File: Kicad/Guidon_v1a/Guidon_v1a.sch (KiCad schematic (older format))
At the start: 0 parts

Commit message: Update Schematic
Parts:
- added C1: 10u, symbol Device:CP1
- added C10, C11, C12, C5, C6, C7, C8, C9: 680n, symbol Device:C
- added C2: 100u, symbol Device:CP1
- added C3, C4: 100n, symbol Device:C
- added D1: D_Schottky_AKA, symbol Device:D_Schottky_AKA
- added IC1: R-785.0-0.5, RECOM_R-785.0-0.5, symbol R-785.0-0.5:R-785.0-0.5
- added IC2: MCP2562, Package_SO:SOIC-8_3.9x4.9mm_P1.27mm, symbol Interface_CAN_LIN:MCP2562-E-SN
- added K1: ALIM, symbol Connector_Generic:Conn_01x02
- added K2: BUS CAN, symbol Connector_Generic:Conn_01x02
- added K3: INTER., symbol Connector_Generic:Conn_01x09
- added K4: OLED, symbol Connector_Generic:Conn_01x04
- added R1: 120, symbol Device:R
- added R10, R2, R3, R4, R5, R6, R7, R8: 6.8k, symbol Device:R
- added R11, R9: 3.3k, symbol Device:R
- added UC1: BluePill STM32, symbol YAAJ_STM32:BluePill_1
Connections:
- new net: IC2.6 (CANL), K2.2 (Pin_2), R1.2
- new net: IC2.7 (CANH), K2.1 (Pin_1), R1.1
- new net: C1.1, D1.2 (K), IC1.1 (+VIN)
- new net: D1.1 (A), D1.3 (A), K1.1 (Pin_1)
- new net +5V: C2.1, C4.2, IC1.3 (+VOUT), IC2.3 (VDD), UC1.18 (5V)
- new net BP0: C5.1, K3.1 (Pin_1), R2.2, UC1.25 (PA0)
- new net BP1: C6.1, K3.2 (Pin_2), R3.2, UC1.26 (PA1)
- new net BP2: C7.1, K3.3 (Pin_3), R4.2, UC1.27 (PA2)
- new net BP3: C8.1, K3.4 (Pin_4), R5.2, UC1.28 (PA3)
- new net BP4: C9.1, K3.5 (Pin_5), R6.2, UC1.29 (PA4)
- new net BP5: C10.1, K3.6 (Pin_6), R7.2, UC1.30 (PA5)
- new net BP6: C11.1, K3.7 (Pin_7), R8.2, UC1.31 (PA6)
- new net BP7: C12.1, K3.8 (Pin_8), R10.2, UC1.32 (PA7)
- new net CANRX: IC2.4 (RXD), UC1.8 (PA11)
- new net CANTX: IC2.1 (TXD), UC1.9 (PA12)
- new net GND: C1.2, C10.2, C11.2, C12.2, C2.2, C3.2, C4.1, C5.2, C6.2, C7.2, C8.2, C9.2, IC1.2 (GND), IC2.2 (VSS), IC2.8 (STBY), K1.2 (Pin_2), K3.9 (Pin_9), K4.2 (Pin_2), UC1.19 (GND), UC1.39 (GND), UC1.40 (GND)
- new net SCL: K4.3 (Pin_3), R11.2, UC1.14 (PB6)
- new net SDA: K4.4 (Pin_4), R9.2, UC1.15 (PB7)
- new net VCC: C3.1, IC2.5 (Vio), K4.1 (Pin_1), R10.1, R11.1, R2.1, R3.1, R4.1, R5.1, R6.1, R7.1, R8.1, R9.1, UC1.20 (3V3)
- no-connect marks 0 -> 23

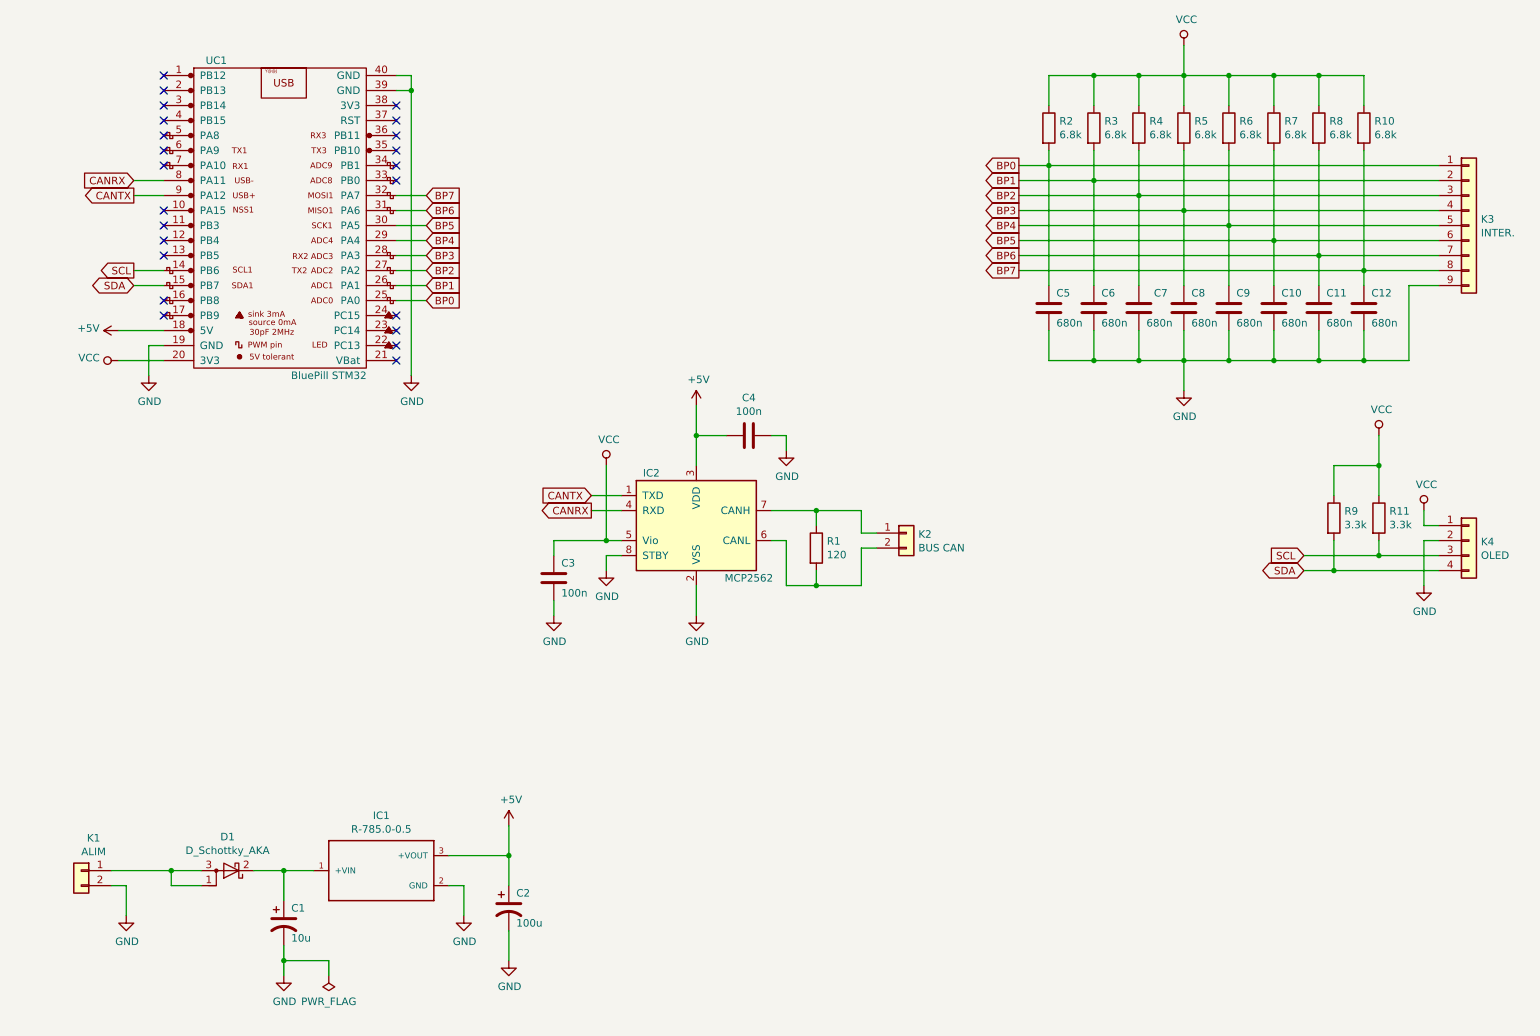
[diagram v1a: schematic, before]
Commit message: Update projet
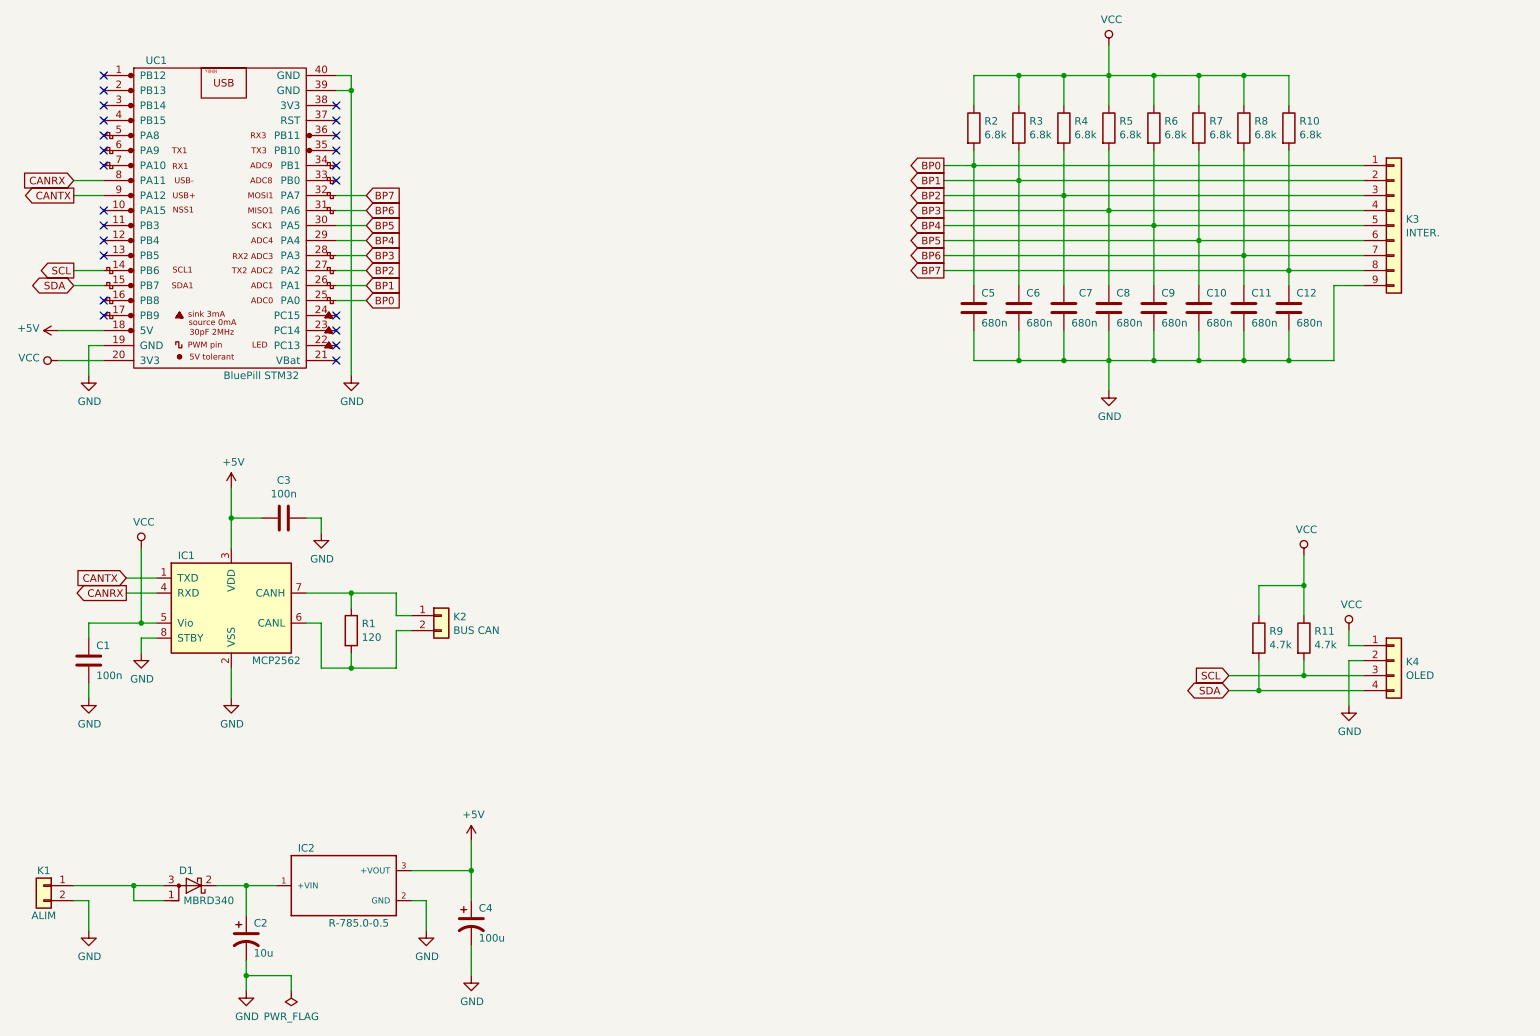
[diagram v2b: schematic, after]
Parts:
- D1: value D_Schottky_AKA -> MBRD340
- R11, R9: value 3.3k -> 4.7k
- renumbered C3 to C1, C1 to C2, C4 to C3, C2 to C4, IC2 to IC1, IC1 to IC2
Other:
- moved on the sheet: C1, C10, C11, C12, C2, C3, C4, C5, C6, C7, C8, C9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

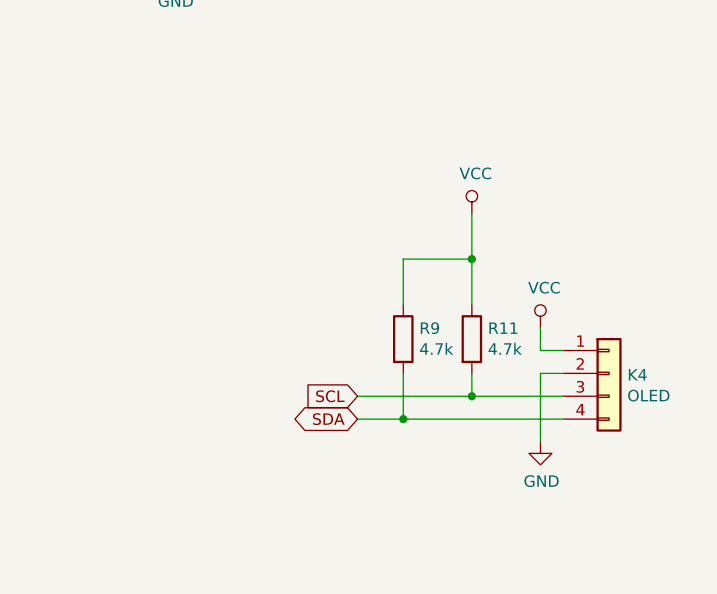
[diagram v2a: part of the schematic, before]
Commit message: Update
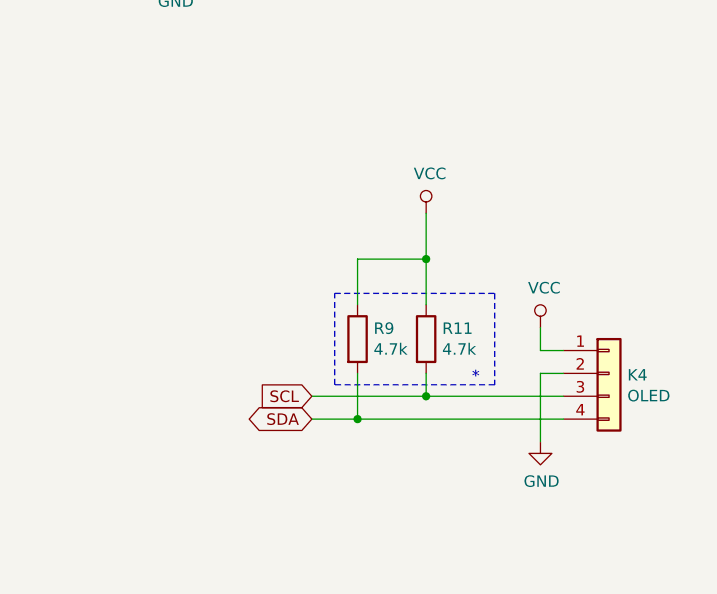
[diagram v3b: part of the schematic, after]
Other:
- note added: "*"
- moved on the sheet: R11, R9
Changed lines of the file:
@@
 Wire Wire Line
 	7200 2400 9200 2400
-Connection ~ 9600 4600
-Wire Wire Line
-	9600 4400 9600 4600
+Connection ~ 9400 4600
+Wire Wire Line
+	9400 4400 9400 4600
 $Comp
 L power:VCC #PWR018
 U 1 1 5E95D1B8
-P 9600 4400
-F 0 "#PWR018" H 9600 4250 50  0001 C CNN
-F 1 "VCC" H 9617 4573 50  0000 C CNN
-F 2 "" H 9600 4400 50  0001 C CNN
-F 3 "" H 9600 4400 50  0001 C CNN
-	1    9600 4400
-	1    0    0    -1
-$EndComp
-Wire Wire Line
-	9600 4600 9600 4800
-Wire Wire Line
-	9300 4600 9600 4600
-Wire Wire Line
-	9300 4800 9300 4600
+P 9400 4400
+F 0 "#PWR018" H 9400 4250 50  0001 C CNN
+F 1 "VCC" H 9417 4573 50  0000 C CNN
+F 2 "" H 9400 4400 50  0001 C CNN
+F 3 "" H 9400 4400 50  0001 C CNN
+	1    9400 4400
+	1    0    0    -1
+$EndComp
+Wire Wire Line
+	9400 4600 9400 4800
+Wire Wire Line
+	9100 4600 9400 4600
+Wire Wire Line
+	9100 4800 9100 4600
 Text GLabel 7200 2500 0    50   Output ~ 0
 BP7
@@
 Wire Wire Line
 	7400 1700 7400 1800
-Text GLabel 9100 5300 0    50   BiDi ~ 0
+Text GLabel 8900 5300 0    50   BiDi ~ 0
 SDA
-Text GLabel 9100 5200 0    50   Input ~ 0
+Text GLabel 8900 5200 0    50   Input ~ 0
 SCL
-Connection ~ 9600 5200
-Wire Wire Line
-	9600 5200 9100 5200
-Connection ~ 9300 5300
-Wire Wire Line
-	9300 5300 9100 5300
-Wire Wire Line
-	9300 5300 9300 5100
-Wire Wire Line
-	10000 5300 9300 5300
-Wire Wire Line
-	9600 5200 9600 5100
-Wire Wire Line
-	10000 5200 9600 5200
-$Comp
-L Device:R R9
-U 1 1 5E8F55B0
-P 9300 4950
-F 0 "R9" H 9370 4996 50  0000 L CNN
-F 1 "4.7k" H 9370 4905 50  0000 L CNN
-F 2 "" V 9230 4950 50  0001 C CNN
-F 3 "~" H 9300 4950 50  0001 C CNN
-	1    9300 4950
-	1    0    0    -1
-$EndComp
+Wire Wire Line
+	9400 5200 8900 5200
+Wire Wire Line
+	9100 5300 8900 5300
+Wire Wire Line
+	9100 5300 9100 5100
+Wire Wire Line
+	9400 5200 9400 5100
 $Comp
 L Device:R R11
 U 1 1 5E8F474D
-P 9600 4950
-F 0 "R11" H 9670 4996 50  0000 L CNN
-F 1 "4.7k" H 9670 4905 50  0000 L CNN
-F 2 "" V 9530 4950 50  0001 C CNN
-F 3 "~" H 9600 4950 50  0001 C CNN
-	1    9600 4950
+P 9400 4950
+F 0 "R11" H 9470 4996 50  0000 L CNN
+F 1 "4.7k" H 9470 4905 50  0000 L CNN
+F 2 "" V 9330 4950 50  0001 C CNN
+F 3 "~" H 9400 4950 50  0001 C CNN
+	1    9400 4950
 	1    0    0    -1
 $EndComp
@@
 $EndComp
 NoConn ~ 3150 1400
+$Comp
+L Device:R R9
+U 1 1 5E8F55B0
+P 9100 4950
+F 0 "R9" H 9170 4996 50  0000 L CNN
+F 1 "4.7k" H 9170 4905 50  0000 L CNN
+F 2 "" V 9030 4950 50  0001 C CNN
+F 3 "~" H 9100 4950 50  0001 C CNN
+	1    9100 4950
+	1    0    0    -1
+$EndComp
+Wire Wire Line
+	10000 5200 9400 5200
+Connection ~ 9400 5200
+Wire Wire Line
+	10000 5300 9100 5300
+Connection ~ 9100 5300
+Wire Notes Line
+	9000 4750 9700 4750
+Wire Notes Line
+	9700 4750 9700 5150
+Wire Notes Line
+	9700 5150 9000 5150
+Wire Notes Line
+	9000 5150 9000 4750
+Text Notes 9600 5150 0    50   ~ 0
+*
 $EndSCHEMATC
